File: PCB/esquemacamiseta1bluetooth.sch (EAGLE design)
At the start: 10 parts

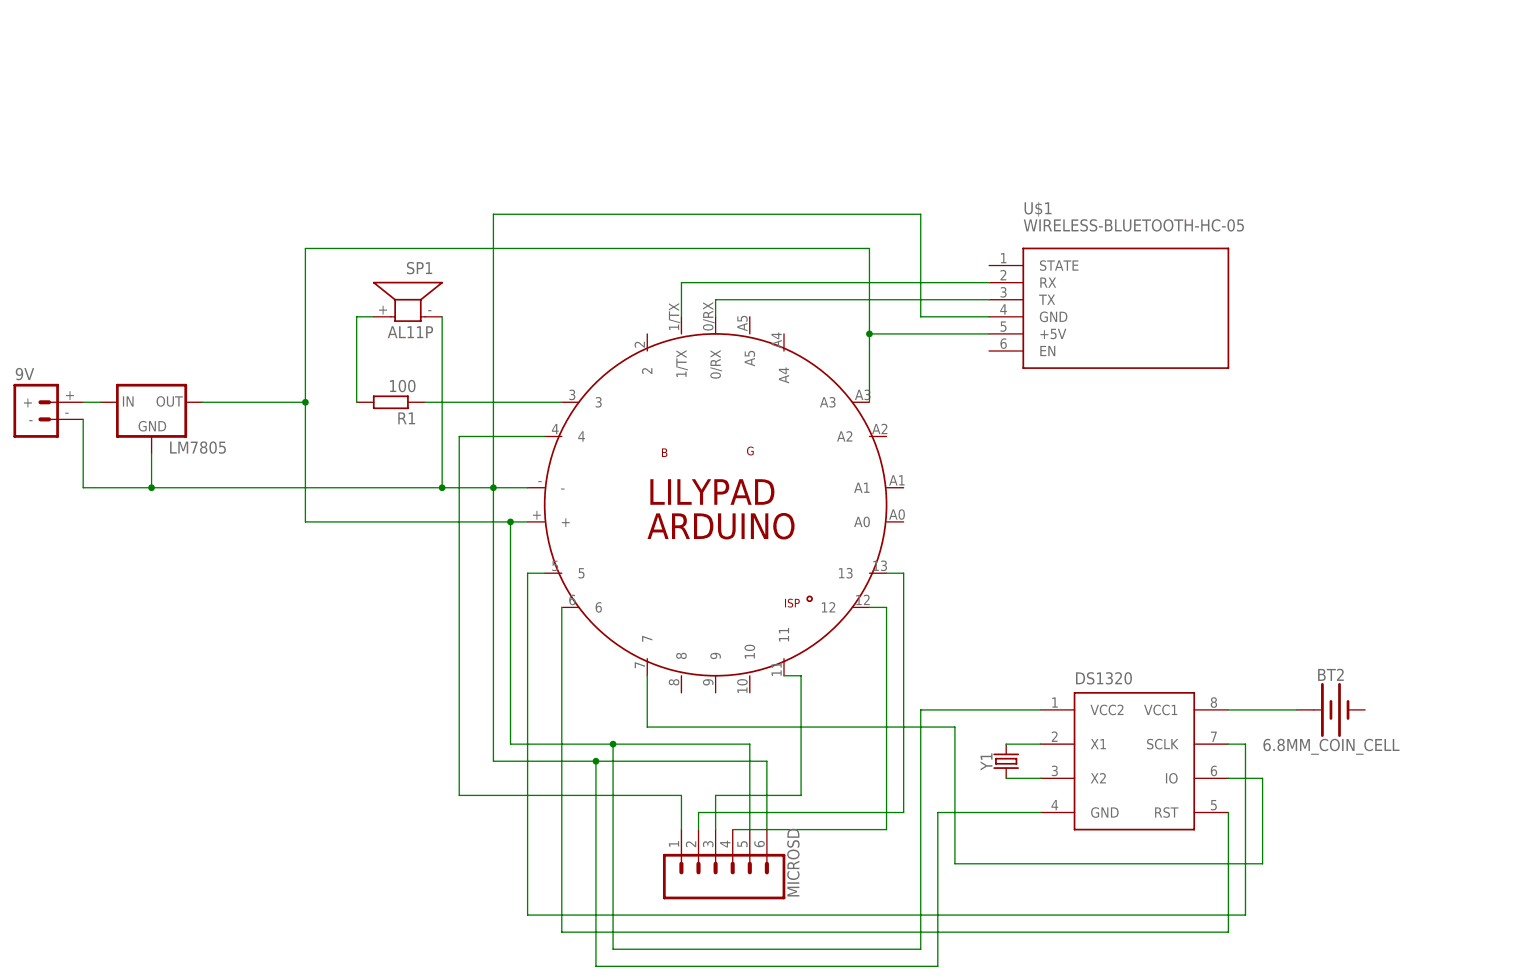
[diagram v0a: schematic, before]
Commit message: Cambios PCB
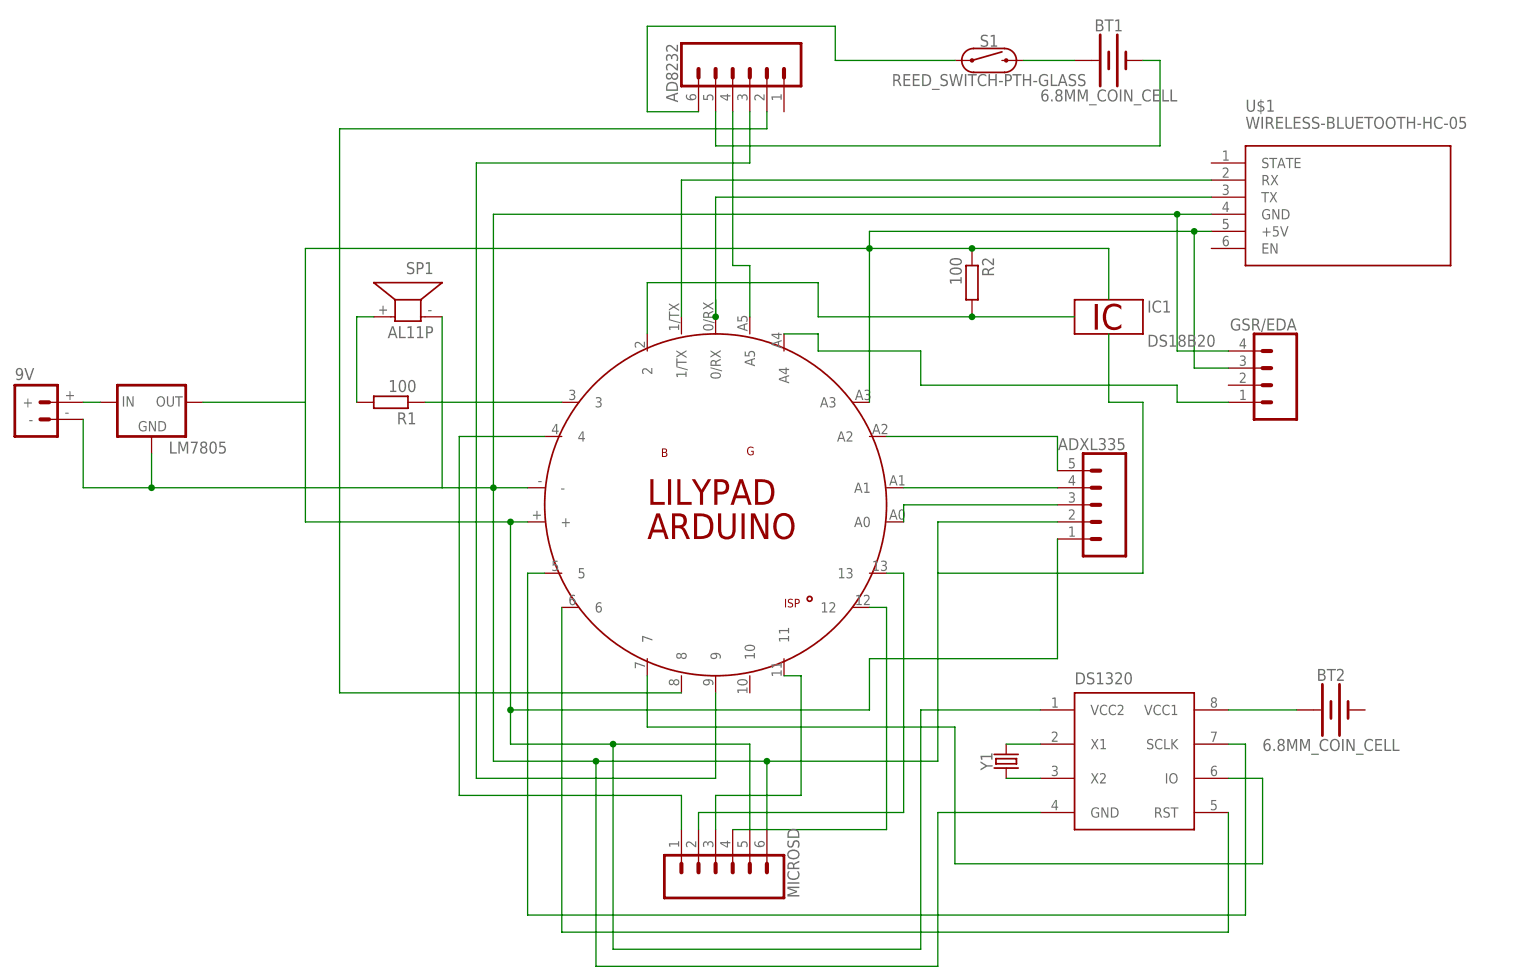
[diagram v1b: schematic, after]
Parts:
- added AD8232: (no value), SparkFun-Connectors:CONN_06FEMALE_LOCK
- added ADXL335: (no value), SparkFun-Connectors:CONN_05
- added BT1: 6.8MM_COIN_CELL, SparkFun-Batteries:BATTERY-6.8MM_SMD
- added GSR/EDA: (no value), SparkFun-Connectors:CONN_04JST-PTH
- added IC1: DS18B20, 1wire:DS18B20
- added R2: 100, rcl:R-EU_0309/12
- added S1: REED_SWITCH-PTH-GLASS, SparkFun-Switches:REED_SWITCH-PTH-GLASS
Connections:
- removed net N$5 (its old number): 9V.-, DS1320.GND, LM7805.GND, MICROSD.6, PCB1.-, SP1.1, U$1.GND
- new net N$19: GSR/EDA.1, PCB1.A4
- new net N$2: LM7805.OUT
- new net N$20: ADXL335.5, PCB1.A2
- new net N$21: ADXL335.4, PCB1.A1
- new net N$22: ADXL335.3, PCB1.A0
- new net N$23: PCB1.2, R2.2
- new net N$24: AD8232.2, PCB1.8
- new net N$25: AD8232.4, PCB1.A5
- new net N$26: AD8232.3, PCB1.9
- new net N$27: BT1.+, S1.2
- new net N$28: AD8232.6, S1.1
- new net N$29: AD8232.5, BT1.-
- new net N$6: 9V.-, ADXL335.2, DS1320.GND, GSR/EDA.4, LM7805.GND, MICROSD.6, PCB1.-, SP1.1, U$1.GND
- net N$3: now also ADXL335.1, GSR/EDA.3, R2.1; no longer LM7805.OUT
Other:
- moved on the sheet: U$1
